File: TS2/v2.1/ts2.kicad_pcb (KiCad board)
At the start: 2 copper layers, 127 x 221 mm, 104 parts, among them P1 FTDI (TERMINAL), P2 FTDI (HOST), P3 +5V POWER, SW1 RESET, SW2 SINGLE STEP/RUN, SW3 STEP, SW4 ABORT, SW5 POWER, U1 555, U10 74LS32, U11 HM6264, U12 28C64, U13 HM6264, U14 28C64, U15 HM6264, U16 28C64, U17 HM6264, U18 28C64, U19 74LS20, U2 8 MHz, U20 74LS74, U21 74LS161, U22 74LS161, U23 74LS74, U24 74LS260, U25 74LS260, U26 74LS138, U27 25LS2548, U28 74LS148, U29 6850, U3 74LS00, U30 6850, U31 MC14411, U32 74LS138, U33 74LS138, U34 74LS00, U35 74LS74, U4 74LS06, U5 74LS04, U6 68000, U7 74LS08, U8 74LS32, U9 74LS32, Y1 1.842MHz

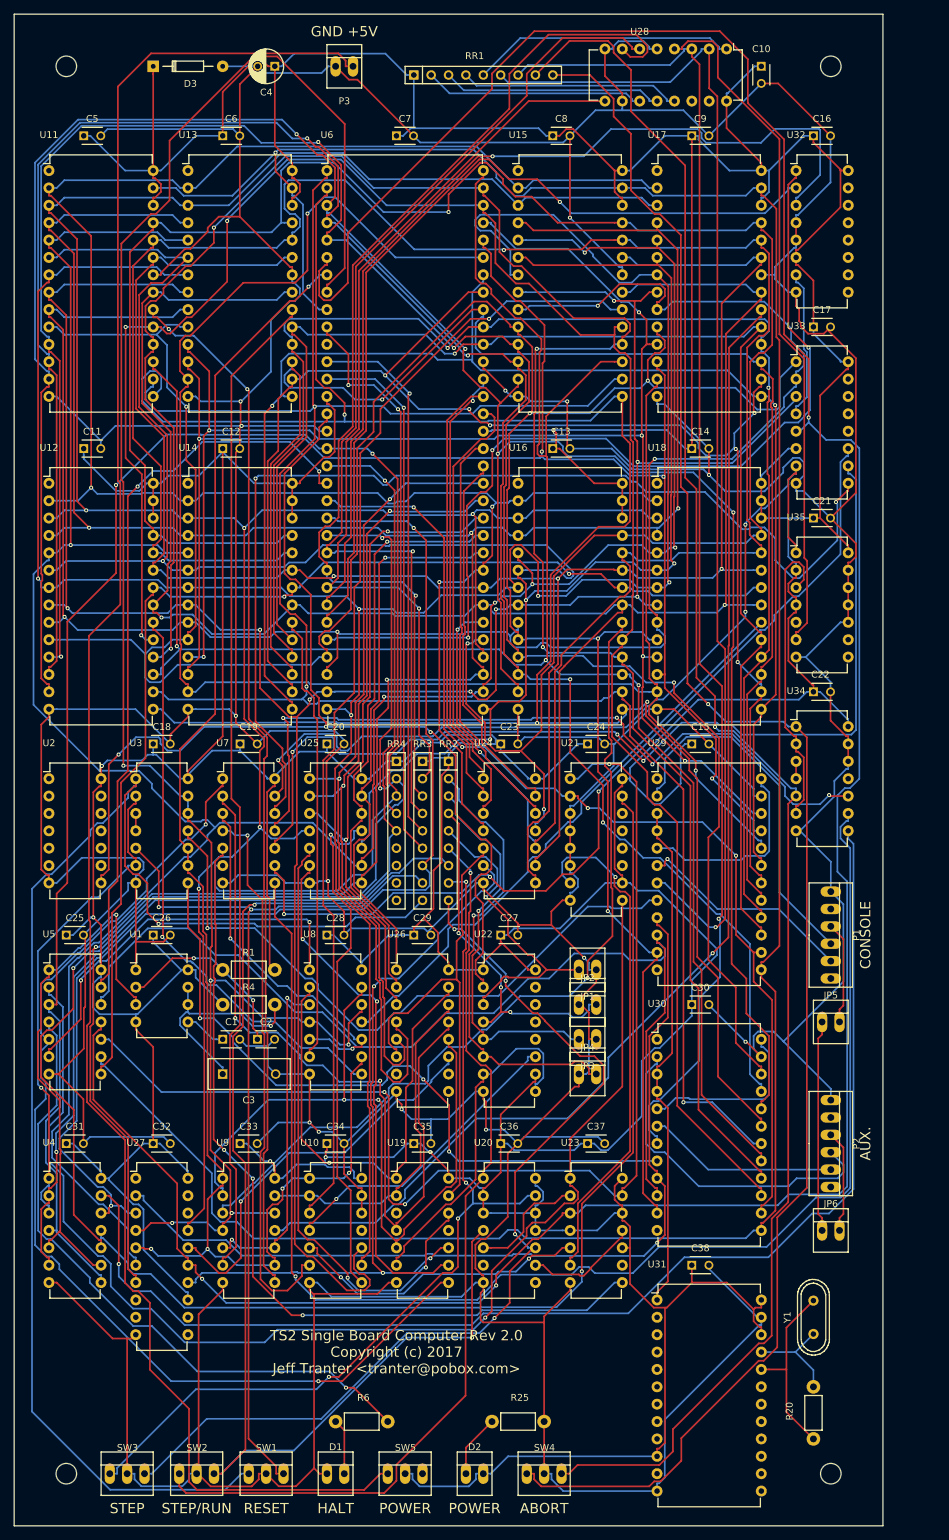
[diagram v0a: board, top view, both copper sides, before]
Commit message: Rev 2.1 design changes.
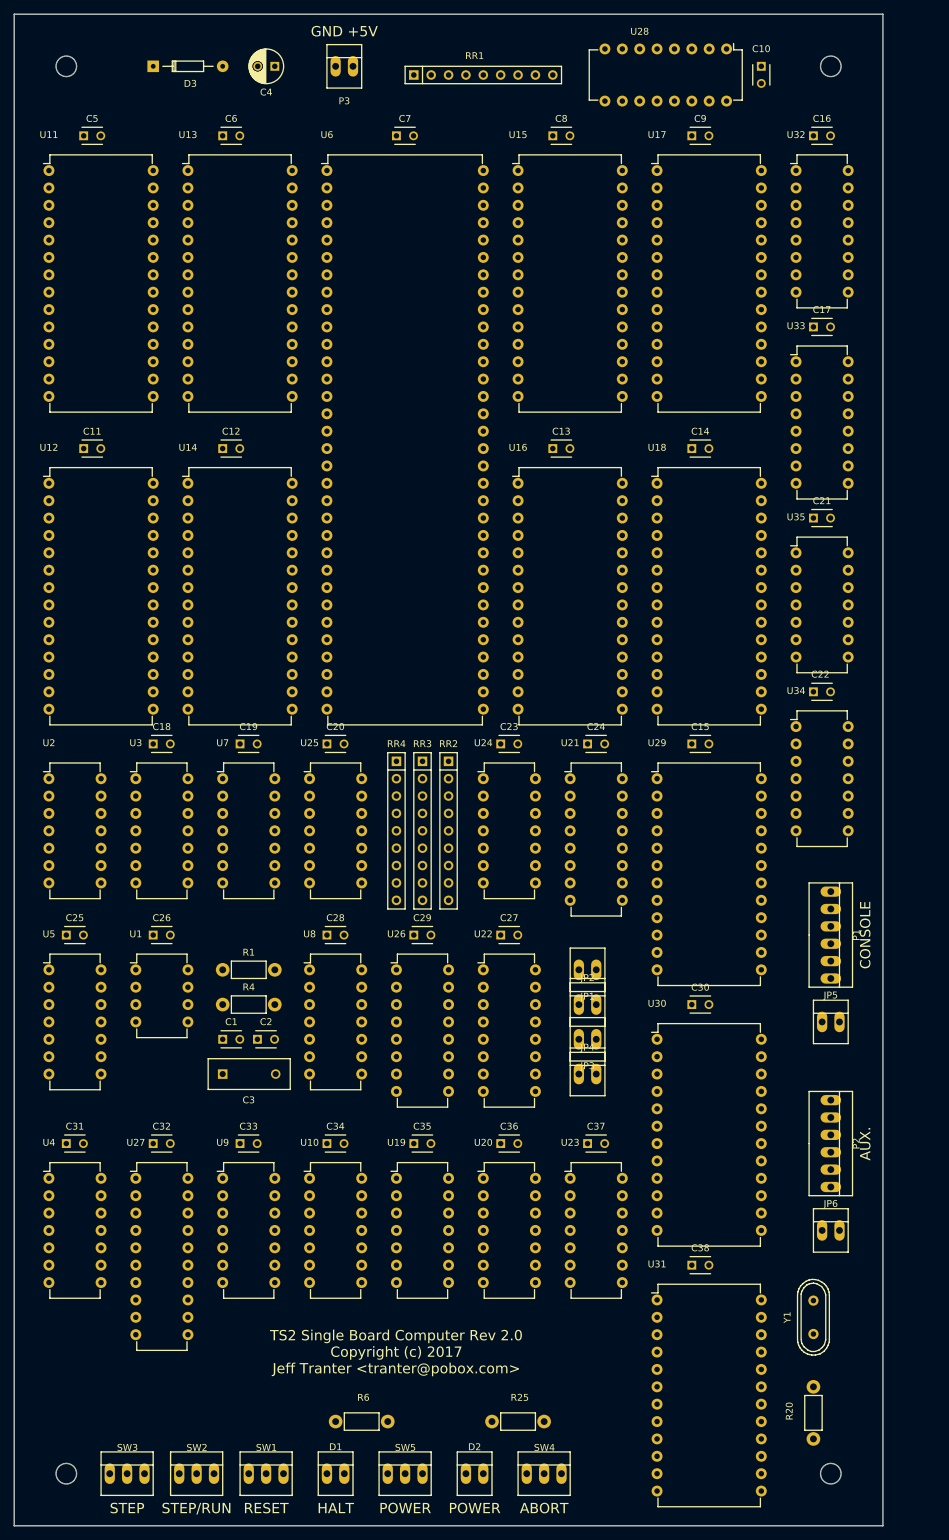
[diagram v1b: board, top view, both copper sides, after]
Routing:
- net GND: track 1424.7 -> 0.00 mm, vias 14 -> 0
- net VCC: track 1296.0 -> 0.00 mm, vias 6 -> 0
- net AS*: track 420.5 -> 0.00 mm, vias 3 -> 0
- net A01: track 412.0 -> 0.00 mm, vias 5 -> 0
- net A06: track 410.3 -> 0.00 mm, vias 6 -> 0
- net R/W*: track 393.6 -> 0.00 mm, vias 1 -> 0
- net A07: track 392.7 -> 0.00 mm, vias 5 -> 0
- net A08: track 378.1 -> 0.00 mm, vias 5 -> 0
- net A03: track 377.4 -> 0.00 mm, vias 8 -> 0
- net A04: track 372.9 -> 0.00 mm, vias 5 -> 0
- net D02: track 353.8 -> 0.00 mm, vias 4 -> 0
- net A10: track 339.3 -> 0.00 mm, vias 3 -> 0
- net A09: track 330.3 -> 0.00 mm, vias 3 -> 0
- net D03: track 321.0 -> 0.00 mm, vias 3 -> 0
- net A05: track 313.4 -> 0.00 mm, vias 4 -> 0
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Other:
- net class Power added: clearance 0.2, trace_width 1, via_dia 0.6, via_drill 0.4

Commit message: Rev 2.1 design changes.
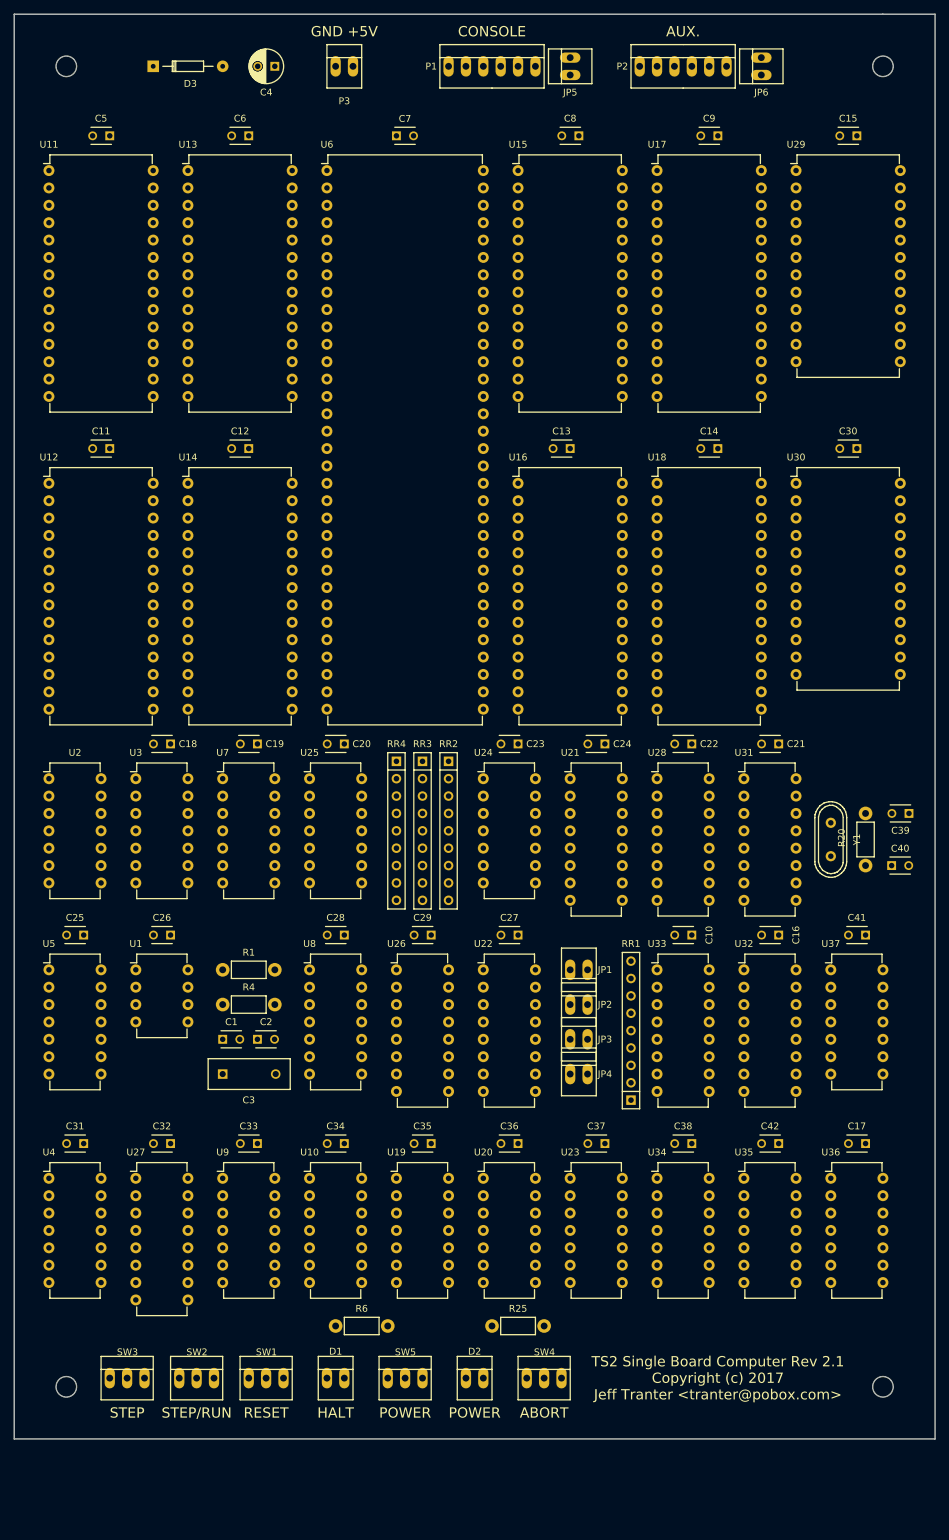
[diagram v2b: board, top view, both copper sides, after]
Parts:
- added C39: 22pF, Capacitors_ThroughHole:C_Disc_D3_P2.5, F.Cu at (153.7, 132.1)
- added C40: 22pF, Capacitors_ThroughHole:C_Disc_D3_P2.5, F.Cu at (151.1, 139.7)
- added C41: 0.1uF, Capacitors_ThroughHole:C_Disc_D3_P2.5, F.Cu at (147.3, 149.9)
- added C42: 0.1uF, Capacitors_ThroughHole:C_Disc_D3_P2.5, F.Cu at (134.6, 180.3)
- added U36: 74LS27, Housings_DIP:DIP-14_W7.62mm, F.Cu at (142.2, 185.4)
- added U37: 74LS00, Housings_DIP:DIP-14_W7.62mm, F.Cu at (142.2, 154.9)
- R20: value 15M -> 10M
- U27: value 25LS2548 -> 74LS138; footprint Housings_DIP:DIP-20_W7.62mm -> Housings_DIP:DIP-16_W7.62mm
- U31: value MC14411 -> 74HC4060; footprint Housings_DIP:DIP-24_W15.24mm -> Housings_DIP:DIP-16_W7.62mm
- Y1: value 1.842MHz -> 2.4576MHz
- moved JP6 170.5 mm to (132.1, 22.9), turned to 90 degrees
- moved P2 159.0 mm to (120.7, 22.9), turned to 0 degrees
- moved JP5 144.8 mm to (104.1, 22.9), turned to 90 degrees
- moved RR1 141.4 mm to (113.0, 163.8), turned to 90 degrees
- moved P1 136.3 mm to (92.7, 22.9), turned to 0 degrees
- moved C10 127.4 mm to (121.9, 149.9), turned to 180 degrees
- moved C17 119.6 mm to (147.3, 180.3), turned to 180 degrees
- moved U32 117.1 mm to (129.5, 154.9)
- moved C16 117.0 mm to (134.6, 149.9), turned to 180 degrees
- moved U28 107.2 mm to (116.8, 127.0), turned to 0 degrees
- moved C15 92.1 mm to (146.1, 33.0), turned to 180 degrees
- moved U35 91.8 mm to (129.5, 185.4)
- moved U29 91.2 mm to (137.2, 38.1)
- moved U33 91.2 mm to (116.8, 154.9)
- moved C30 84.8 mm to (146.1, 78.7), turned to 180 degrees
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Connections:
- R20 pad 1: Net-(R20-Pad1) -> Net-(C40-Pad1)
- R20 pad 2: Net-(R20-Pad2) -> Net-(C39-Pad2)
- U27 pad 1: Net-(U27-Pad1) -> A06
- U27 pad 10: GND -> Net-(U27-Pad10)
- U27 pad 13: VCC -> Net-(U27-Pad13)
- U27 pad 14: Net-(U19-Pad10) -> CS_PERI2*
- U27 pad 15: AS* -> Net-(U27-Pad15)
- U27 pad 16: Net-(U26-Pad11) -> VCC
- U27 pad 2: CS_PERI2* -> A07
- U27 pad 3: VPA* -> A08
- U27 pad 4: UDS* -> Net-(U26-Pad11)
- U27 pad 5: LDS* -> AS*
- U27 pad 6: A06 -> Net-(U19-Pad10)
- U27 pad 7: A07 -> Net-(U27-Pad7)
- U27 pad 8: Net-(U27-Pad8) -> GND
- U31 pad 1: Net-(U29-Pad3) -> Net-(U31-Pad1)
- U31 pad 10: VCC -> Net-(C40-Pad1)
- U31 pad 11: (no net) -> Net-(C39-Pad2)
- U31 pad 13: (no net) -> Net-(U31-Pad13)
- U31 pad 14: (no net) -> Net-(U31-Pad14)
- U31 pad 15: (no net) -> Net-(U31-Pad15)
- U31 pad 16: (no net) -> VCC
- U31 pad 6: (no net) -> Net-(U31-Pad6)
- U31 pad 7: Net-(U31-Pad7) -> Net-(U29-Pad3)
- U31 pad 8: (no net) -> GND
- U31 pad 9: (no net) -> Net-(U31-Pad9)
- U34 pad 12: GND -> Net-(U34-Pad12)
- U34 pad 13: GND -> PERI_VPA*
- U4 pad 13: Net-(U34-Pad8) -> Net-(U34-Pad11)
- Y1 pad 1: Net-(R20-Pad2) -> Net-(C39-Pad2)
- Y1 pad 2: Net-(R20-Pad1) -> Net-(C40-Pad1)
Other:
- board size 127 x 221 mm -> 134.6 x 208.3 mm
- board text added: "TS2 Single Board Computer Rev 2.1 Copyright (c) 2017 Jeff Tranter <tranter@pobox.com>"
- board text removed: "TS2 Single Board Computer Rev 2.0 Copyright (c) 2017 Jeff Tranter <tranter@pobox.com>"

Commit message: Import PCB layout.
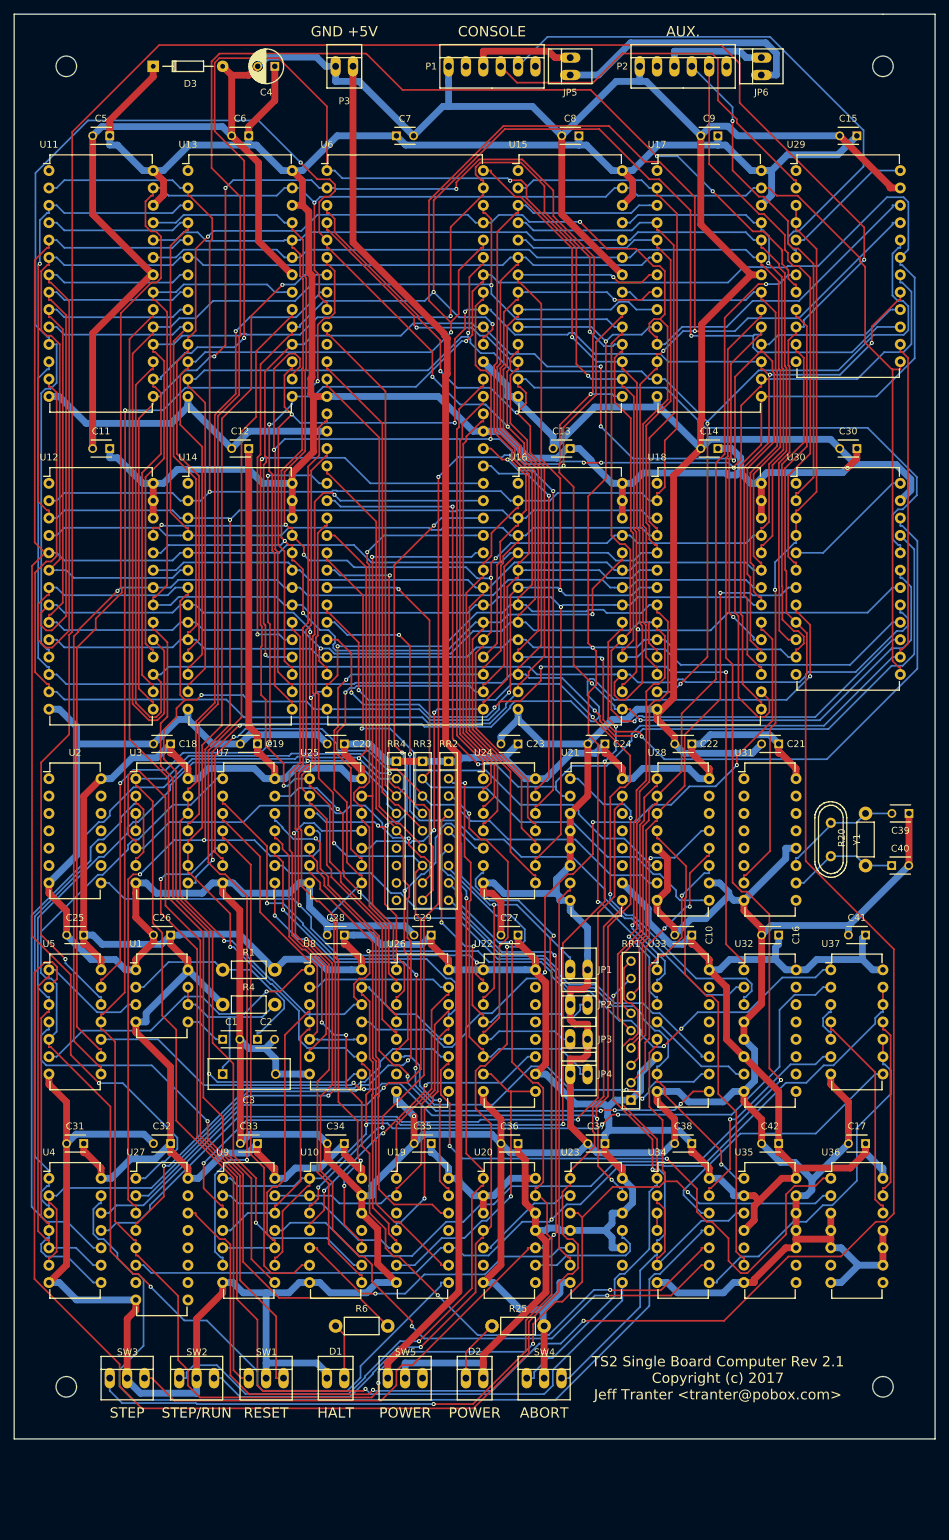
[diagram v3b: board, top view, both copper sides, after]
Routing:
- net GND: track 0.00 -> 1388.1 mm, vias 0 -> 1
- net VCC: track 0.00 -> 1108.4 mm, vias 0 -> 1
- net A03: track 0.00 -> 412.1 mm, vias 0 -> 7
- net A06: track 0.00 -> 409.9 mm, vias 0 -> 2
- net A08: track 0.00 -> 387.8 mm, vias 0 -> 4
- net A04: track 0.00 -> 387.7 mm, vias 0 -> 5
- net A07: track 0.00 -> 374.7 mm, vias 0 -> 3
- net A01: track 0.00 -> 354.4 mm, vias 0 -> 3
- net AS*: track 0.00 -> 342.8 mm, vias 0 -> 5
- net Net-(U29-Pad10): track 0.00 -> 336.8 mm, vias 0 -> 2
- net R/W*: track 0.00 -> 329.9 mm, vias 0 -> 1
- net D00: track 0.00 -> 324.5 mm, vias 0 -> 5
- net A10: track 0.00 -> 316.0 mm, vias 0 -> 3
- net A02: track 0.00 -> 298.2 mm, vias 0 -> 2
- net D02: track 0.00 -> 294.9 mm, vias 0 -> 2
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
